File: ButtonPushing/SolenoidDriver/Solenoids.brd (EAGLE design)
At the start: 20.3 x 43.2 mm, 29 parts, among them U1 TLE94112EL

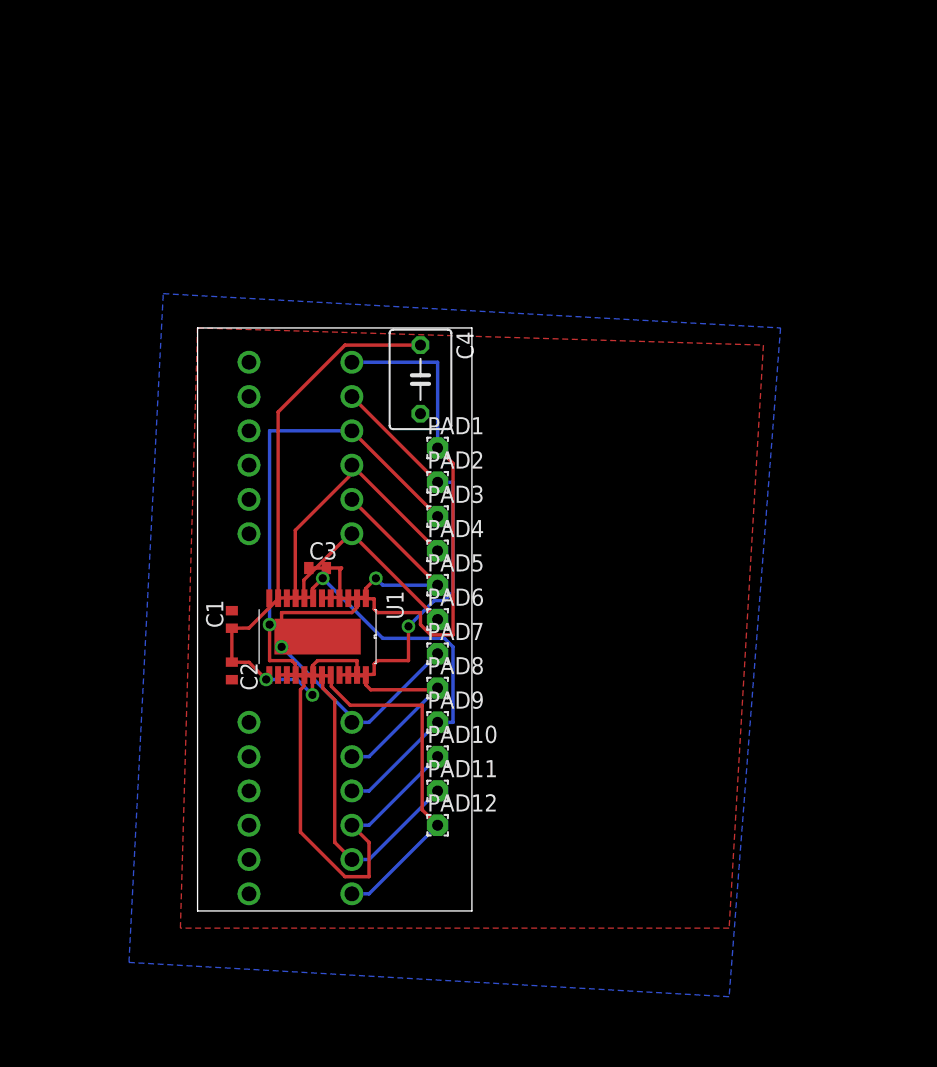
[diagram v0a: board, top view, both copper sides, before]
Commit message: Fully routed PCB
Basically done, but needs to be checked over
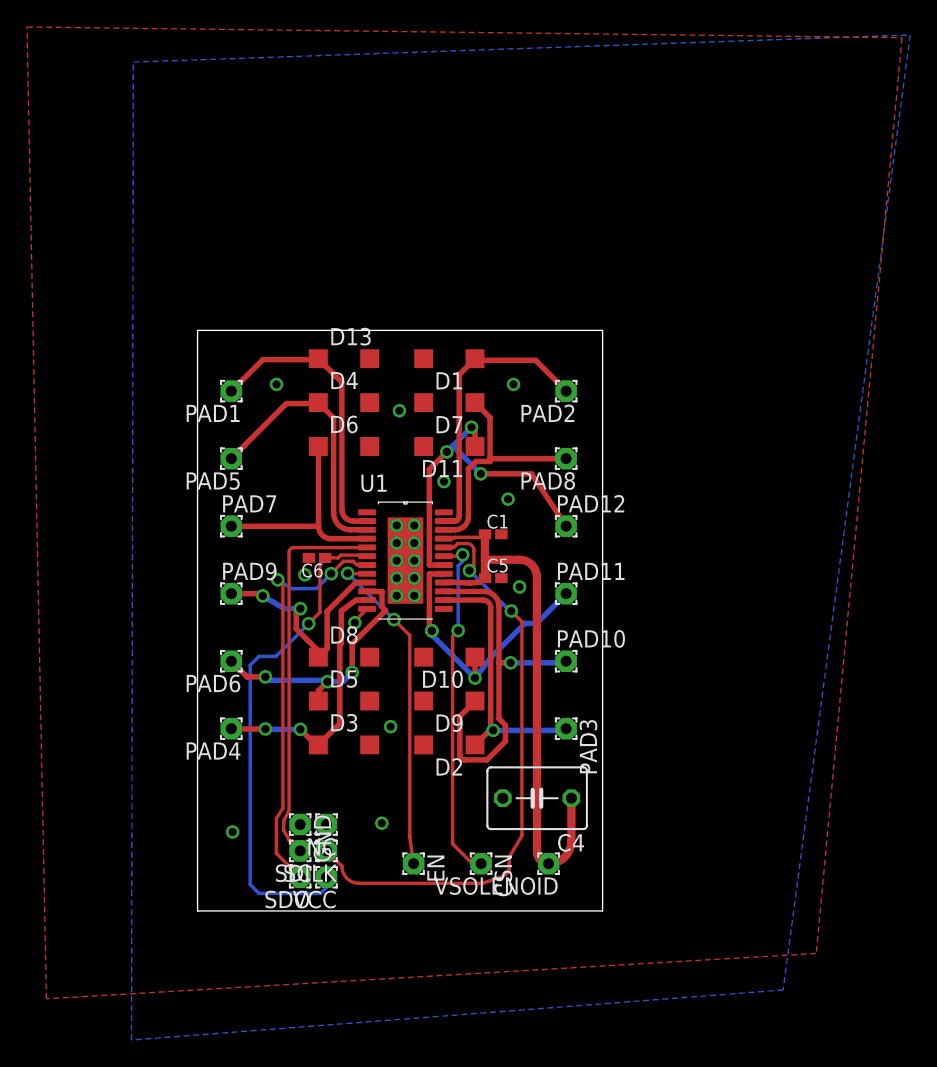
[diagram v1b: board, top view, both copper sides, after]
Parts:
- removed C2, C3: 100nF, rcl:C0402
- removed D12: 1N5819-B, diode:DO41-7.6
- added C5, C6: 100nF, rcl:C0402K
- added CSN, EN, GND, NC, SCLK, SDI, SDO, VCC, VSOLENOID: (no value), wirepad:1,6/0,8
- added D13: MBR0520LT, diode:SOD123
- C1: device rcl:C0402 -> rcl:C0402K
- D1, D10, D11, D2, D3, D4, D5, D6, D7, D8, D9: value 1N5819-B -> MBR0520LT; device diode:DO41-7.6 -> diode:SOD123
- moved D11 32.5 mm to (18.6, 34.4), flipped to the top, turned to 180 degrees
- moved C4 32.2 mm to (25.1, 8.35), turned to 180 degrees
- moved D2 28.1 mm to (18.6, 12.3), flipped to the top, turned to 180 degrees
- moved D7 26.1 mm to (18.6, 37.6), flipped to the top, turned to 180 degrees
- moved PAD12 24.1 mm to (27.3, 28.5)
- moved D3 23.5 mm to (10.8, 12.3), flipped to the top
- moved C1 20.4 mm to (21.9, 27.9), turned to 0 degrees
- moved PAD4 20.2 mm to (2.50, 13.5), turned to 180 degrees
- moved PAD8 19.5 mm to (27.3, 33.5), turned to 180 degrees
- moved PAD3 18.4 mm to (27.3, 13.5), turned to 270 degrees
- moved PAD9 18.0 mm to (2.50, 23.5)
- moved PAD7 18.0 mm to (2.50, 28.5)
- moved PAD5 17.9 mm to (2.50, 33.5), turned to 180 degrees
- moved PAD11 17.4 mm to (27.3, 23.5)
- moved D10 16.6 mm to (18.6, 18.8), flipped to the top, turned to 180 degrees
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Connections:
- removed net CS: U1.19
- removed net EN: U1.8
- removed net MISO: U1.7
- removed net MOSI: U1.5
- removed net SCK: U1.20
- removed net SOLENOID: C1.1, C2.1, C4.1, U1.16, U1.21
- new net N$22: EN.1, U1.8
- new net N$23: CSN.1, U1.19
- new net N$24: SCLK.1, U1.20
- new net N$25: SDI.1, U1.5
- new net N$26: SDO.1, U1.7
- new net VDD: C1.1, C4.1, C5.1, U1.16, U1.21, VSOLENOID.1
- net GND: now also C5.2, C6.2, D13.A, GND.1, NC.1; no longer C2.2, C3.2, D12.A
- net N$1: now also D13.C; no longer D1.C
- net N$10: now also D9.C; no longer D10.C
- net N$11: now also D10.C; no longer D11.C
- net N$12: now also D11.C; no longer D12.C
- net N$2: now also D1.C; no longer D2.C
- net N$3: now also D2.C; no longer D3.C
- net N$4: now also D3.C; no longer D4.C
- net N$5: now also D4.C; no longer D5.C
- net N$6: now also D5.C; no longer D6.C
- net N$7: now also D6.C; no longer D7.C
- net N$8: now also D7.C; no longer D8.C
- net N$9: now also D8.C; no longer D9.C
- net VCC: now also C6.1, VCC.1; no longer C3.1
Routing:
- net SOLENOID: track 50.5 -> 0.00 mm, vias 2 -> 0
- net N$24: track 0.00 -> 43.0 mm, vias 0 -> 2
- net VDD: track 0.00 -> 41.4 mm
- net VCC: track 5.97 -> 37.3 mm, vias 0 -> 1
- net N$26: track 0.00 -> 30.8 mm, vias 0 -> 2
- net N$25: track 0.00 -> 28.6 mm
- net N$23: track 0.00 -> 26.1 mm, vias 0 -> 2
- net N$22: track 0.00 -> 24.9 mm, vias 0 -> 2
- net N$3: track 36.1 -> 20.0 mm
- net N$1: track 36.2 -> 21.5 mm
- net N$9: track 29.9 -> 17.4 mm, vias 1 -> 2
- net N$7: track 26.6 -> 16.4 mm, vias 1 -> 0
- net N$2: track 29.8 -> 21.2 mm, vias 1 -> 0
- net N$10: track 32.2 -> 28.3 mm, vias 0 -> 1
- net N$6: track 16.6 -> 19.8 mm, vias 0 -> 3
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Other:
- board size 20.3 x 43.2 mm -> 30 x 43 mm
- board text added: "#0"
- board text added: "#1"
- board text added: "#10"
- board text added: "#11"
- board text added: "#2"
- board text added: "#3"
- board text added: "#4"
- board text added: "#5"
- board text added: "#6"
- board text added: "#7"
- board text added: "#8"
- board text added: "#9"
- board text added: "100nF"
- board text added: "47uF"
- board text added: "CSN"
- board text added: "EN"
- board text added: "GND"
- board text added: "Instructions: Connect the VSolenoid to all the solenoids and connect each solenoid's ground wire to its respective numbered terminal"
- board text added: "NC"
- board text added: "SCLK"
- board text added: "SDI"
- board text added: "SDO"
- board text added: "Solenoid Driver Board 2020 Using TLE94112EL For CAR by William Daniels Based off of schematic from TLE94112EL Motor Shield"
- board text added: "VCC"
- board text added: "VSolenoid"
